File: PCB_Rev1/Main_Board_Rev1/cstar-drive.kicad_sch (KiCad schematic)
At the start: 2 parts, among them J12 532610771, J9 532610771

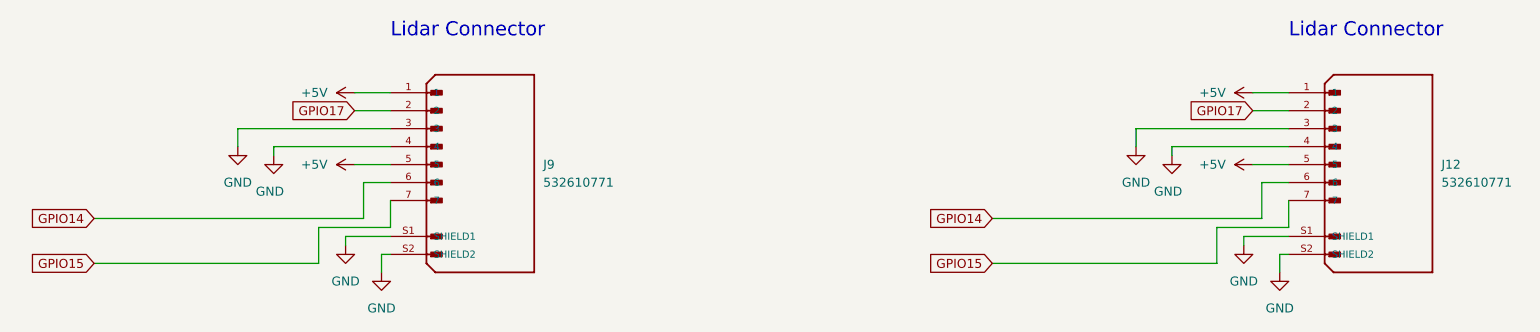
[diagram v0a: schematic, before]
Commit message: Audio Back
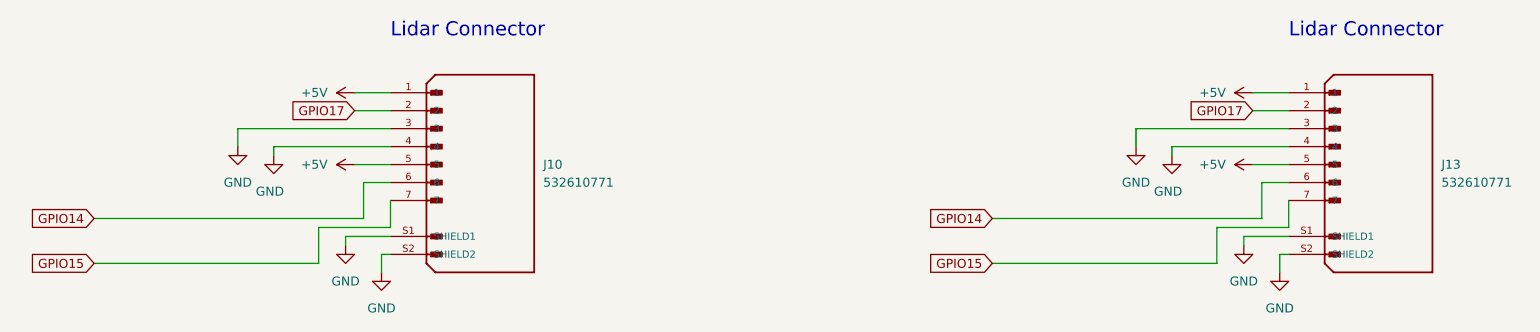
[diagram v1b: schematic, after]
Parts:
- renumbered J9 to J10, J12 to J13
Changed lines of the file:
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@@
 		(dnp no)
 		(fields_autoplaced yes)
-		(property "Reference" "#PWR038"
+		(property "Reference" "#PWR049"
 			(at 97.79 88.9 0)
 			(effects
@@
 					(unit 1)
 				)
-				(path "/8f5a23de-a1fa-4202-92fb-c2ac3de0338c/b82e2994-3828-4951-9572-d8060e0d0a41"
-					(reference "#PWR038")
-					(unit 1)
-				)
 			)
 		)
@@
 		(dnp no)
 		(fields_autoplaced yes)
-		(property "Reference" "J9"
+		(property "Reference" "J10"
 			(at 120.65 88.9 0)
 			(effects
@@
 					(unit 1)
 				)
-				(path "/8f5a23de-a1fa-4202-92fb-c2ac3de0338c/b82e2994-3828-4951-9572-d8060e0d0a41"
-					(reference "J9")
-					(unit 1)
-				)
 			)
 		)
@@
 		(dnp no)
 		(fields_autoplaced yes)
-		(property "Reference" "#PWR056"
+		(property "Reference" "#PWR062"
 			(at 224.79 110.49 0)
 			(effects
@@
 					(unit 1)
 				)
-				(path "/8f5a23de-a1fa-4202-92fb-c2ac3de0338c/b82e2994-3828-4951-9572-d8060e0d0a41"
-					(reference "#PWR056")
-					(unit 1)
-				)
 			)
 		)
@@
 		(dnp no)
 		(fields_autoplaced yes)
-		(property "Reference" "#PWR036"
+		(property "Reference" "#PWR047"
 			(at 92.71 106.68 0)
 			(effects
@@
 					(unit 1)
 				)
-				(path "/8f5a23de-a1fa-4202-92fb-c2ac3de0338c/b82e2994-3828-4951-9572-d8060e0d0a41"
-					(reference "#PWR036")
-					(unit 1)
-				)
 			)
 		)
@@
 		(dnp no)
 		(fields_autoplaced yes)
-		(property "Reference" "#PWR055"
+		(property "Reference" "#PWR061"
 			(at 224.79 88.9 0)
 			(effects
@@
 					(unit 1)
 				)
-				(path "/8f5a23de-a1fa-4202-92fb-c2ac3de0338c/b82e2994-3828-4951-9572-d8060e0d0a41"
-					(reference "#PWR055")
-					(unit 1)
-				)
 			)
 		)
@@
 		(dnp no)
 		(fields_autoplaced yes)
-		(property "Reference" "#PWR037"
+		(property "Reference" "#PWR048"
 			(at 97.79 78.74 0)
 			(effects
@@
 					(unit 1)
 				)
-				(path "/8f5a23de-a1fa-4202-92fb-c2ac3de0338c/b82e2994-3828-4951-9572-d8060e0d0a41"
-					(reference "#PWR037")
-					(unit 1)
-				)
 			)
 		)
@@
 		(dnp no)
 		(fields_autoplaced yes)
-		(property "Reference" "#PWR054"
+		(property "Reference" "#PWR060"
 			(at 224.79 78.74 0)
 			(effects
@@
 					(unit 1)
 				)
-				(path "/8f5a23de-a1fa-4202-92fb-c2ac3de0338c/b82e2994-3828-4951-9572-d8060e0d0a41"
-					(reference "#PWR054")
-					(unit 1)
-				)
 			)
 		)
@@
 		(dnp no)
 		(fields_autoplaced yes)
-		(property "Reference" "#PWR051"
+		(property "Reference" "#PWR057"
 			(at 204.47 92.71 0)
 			(effects
@@
 					(unit 1)
 				)
-				(path "/8f5a23de-a1fa-4202-92fb-c2ac3de0338c/b82e2994-3828-4951-9572-d8060e0d0a41"
-					(reference "#PWR051")
-					(unit 1)
-				)
 			)
 		)
@@
 		(on_board yes)
 		(dnp no)
-		(property "Reference" "#PWR035"
+		(property "Reference" "#PWR046"
 			(at 82.55 93.98 0)
 			(effects
@@
 					(unit 1)
 				)
-				(path "/8f5a23de-a1fa-4202-92fb-c2ac3de0338c/b82e2994-3828-4951-9572-d8060e0d0a41"
-					(reference "#PWR035")
-					(unit 1)
-				)
 			)
 		)
@@
 		(dnp no)
 		(fields_autoplaced yes)
-		(property "Reference" "#PWR053"
+		(property "Reference" "#PWR059"
 			(at 219.71 106.68 0)
 			(effects
@@
 					(unit 1)
 				)
-				(path "/8f5a23de-a1fa-4202-92fb-c2ac3de0338c/b82e2994-3828-4951-9572-d8060e0d0a41"
-					(reference "#PWR053")
-					(unit 1)
-				)
 			)
 		)
@@
 		(on_board yes)
 		(dnp no)
-		(property "Reference" "#PWR052"
+		(property "Reference" "#PWR058"
 			(at 209.55 93.98 0)
 			(effects
@@
 					(unit 1)
 				)
-				(path "/8f5a23de-a1fa-4202-92fb-c2ac3de0338c/b82e2994-3828-4951-9572-d8060e0d0a41"
-					(reference "#PWR052")
-					(unit 1)
-				)
 			)
 		)
@@
 		(dnp no)
 		(fields_autoplaced yes)
-		(property "Reference" "J12"
+		(property "Reference" "J13"
 			(at 247.65 88.9 0)
 			(effects
@@
 					(unit 1)
 				)
-				(path "/8f5a23de-a1fa-4202-92fb-c2ac3de0338c/b82e2994-3828-4951-9572-d8060e0d0a41"
-					(reference "J12")
-					(unit 1)
-				)
 			)
 		)
@@
 		(dnp no)
 		(fields_autoplaced yes)
-		(property "Reference" "#PWR034"
+		(property "Reference" "#PWR045"
 			(at 77.47 92.71 0)
 			(effects
@@
 					(unit 1)
 				)
-				(path "/8f5a23de-a1fa-4202-92fb-c2ac3de0338c/b82e2994-3828-4951-9572-d8060e0d0a41"
-					(reference "#PWR034")
-					(unit 1)
-				)
 			)
 		)
@@
 		(dnp no)
 		(fields_autoplaced yes)
-		(property "Reference" "#PWR039"
+		(property "Reference" "#PWR050"
 			(at 97.79 110.49 0)
 			(effects
@@
 					(unit 1)
 				)
-				(path "/8f5a23de-a1fa-4202-92fb-c2ac3de0338c/b82e2994-3828-4951-9572-d8060e0d0a41"
-					(reference "#PWR039")
-					(unit 1)
-				)
